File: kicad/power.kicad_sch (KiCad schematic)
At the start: 30 parts, among them J3 Conn_01x02, P1 USB_C_Plug_USB2.0, Q1 BCW66G, Q2 BCW66G, U3 TP4056-42-ESOP8, U4 U8205A, U5 DW01A, U6 USBLC6-2P6, U7 CH340C, U8 AMS1117-3.3

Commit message: init
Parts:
- R10, R11, R12, R3, R4, R5, R6, R7, R8, R9: footprint Resistor_SMD:R_0805_2012Metric -> Resistor_SMD:R_1206_3216Metric
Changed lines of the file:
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@@
 			)
 		)
-		(property "Footprint" "Resistor_SMD:R_0805_2012Metric"
+		(property "Footprint" "Resistor_SMD:R_1206_3216Metric"
 			(at 85.598 163.83 90)
 			(effects
@@
 			)
 		)
-		(property "Footprint" "Resistor_SMD:R_0805_2012Metric"
+		(property "Footprint" "Resistor_SMD:R_1206_3216Metric"
 			(at 105.918 162.56 90)
 			(effects
@@
 			)
 		)
-		(property "Footprint" "Resistor_SMD:R_0805_2012Metric"
+		(property "Footprint" "Resistor_SMD:R_1206_3216Metric"
 			(at 150.368 130.81 90)
 			(effects
@@
 			)
 		)
-		(property "Footprint" "Resistor_SMD:R_0805_2012Metric"
+		(property "Footprint" "Resistor_SMD:R_1206_3216Metric"
 			(at 114.808 154.94 90)
 			(effects
@@
 			)
 		)
-		(property "Footprint" "Resistor_SMD:R_0805_2012Metric"
+		(property "Footprint" "Resistor_SMD:R_1206_3216Metric"
 			(at 105.918 139.7 90)
 			(effects
@@
 			)
 		)
-		(property "Footprint" "Resistor_SMD:R_0805_2012Metric"
+		(property "Footprint" "Resistor_SMD:R_1206_3216Metric"
 			(at 32.258 147.32 90)
 			(effects
@@
 			)
 		)
-		(property "Footprint" "Resistor_SMD:R_0805_2012Metric"
+		(property "Footprint" "Resistor_SMD:R_1206_3216Metric"
 			(at 222.25 79.248 90)
 			(effects
@@
 			)
 		)
-		(property "Footprint" "Resistor_SMD:R_0805_2012Metric"
+		(property "Footprint" "Resistor_SMD:R_1206_3216Metric"
 			(at 221.742 35.56 90)
 			(effects
@@
 			)
 		)
-		(property "Footprint" "Resistor_SMD:R_0805_2012Metric"
+		(property "Footprint" "Resistor_SMD:R_1206_3216Metric"
 			(at 222.25 100.838 90)
 			(effects
@@
 			)
 		)
-		(property "Footprint" "Resistor_SMD:R_0805_2012Metric"
+		(property "Footprint" "Resistor_SMD:R_1206_3216Metric"
 			(at 47.498 147.32 90)
 			(effects

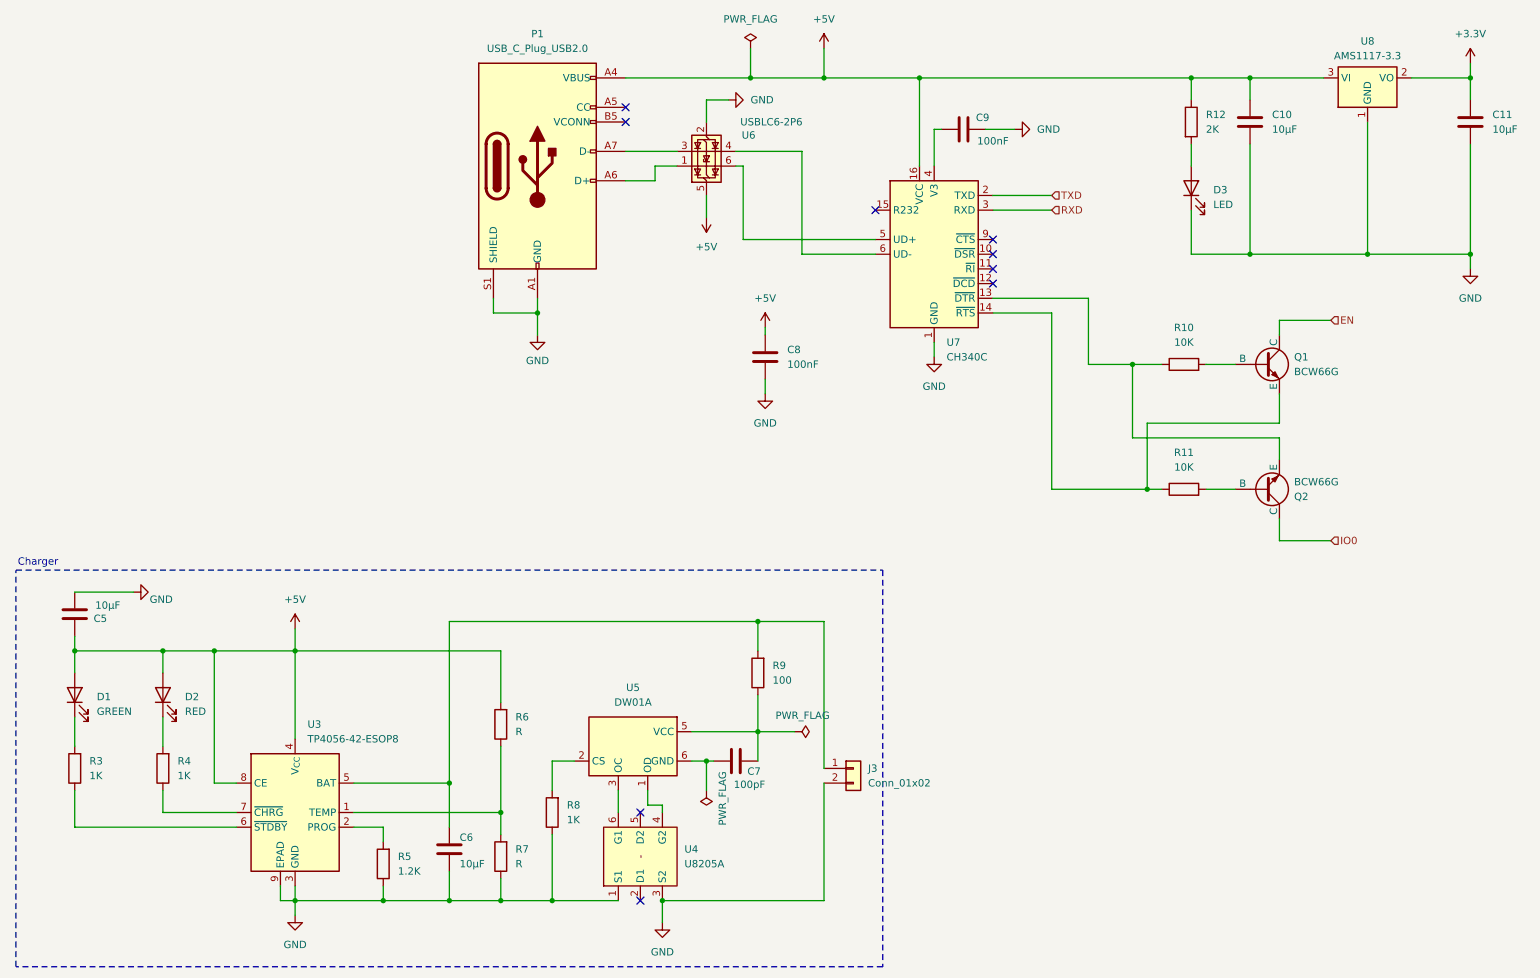
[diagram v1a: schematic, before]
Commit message: init
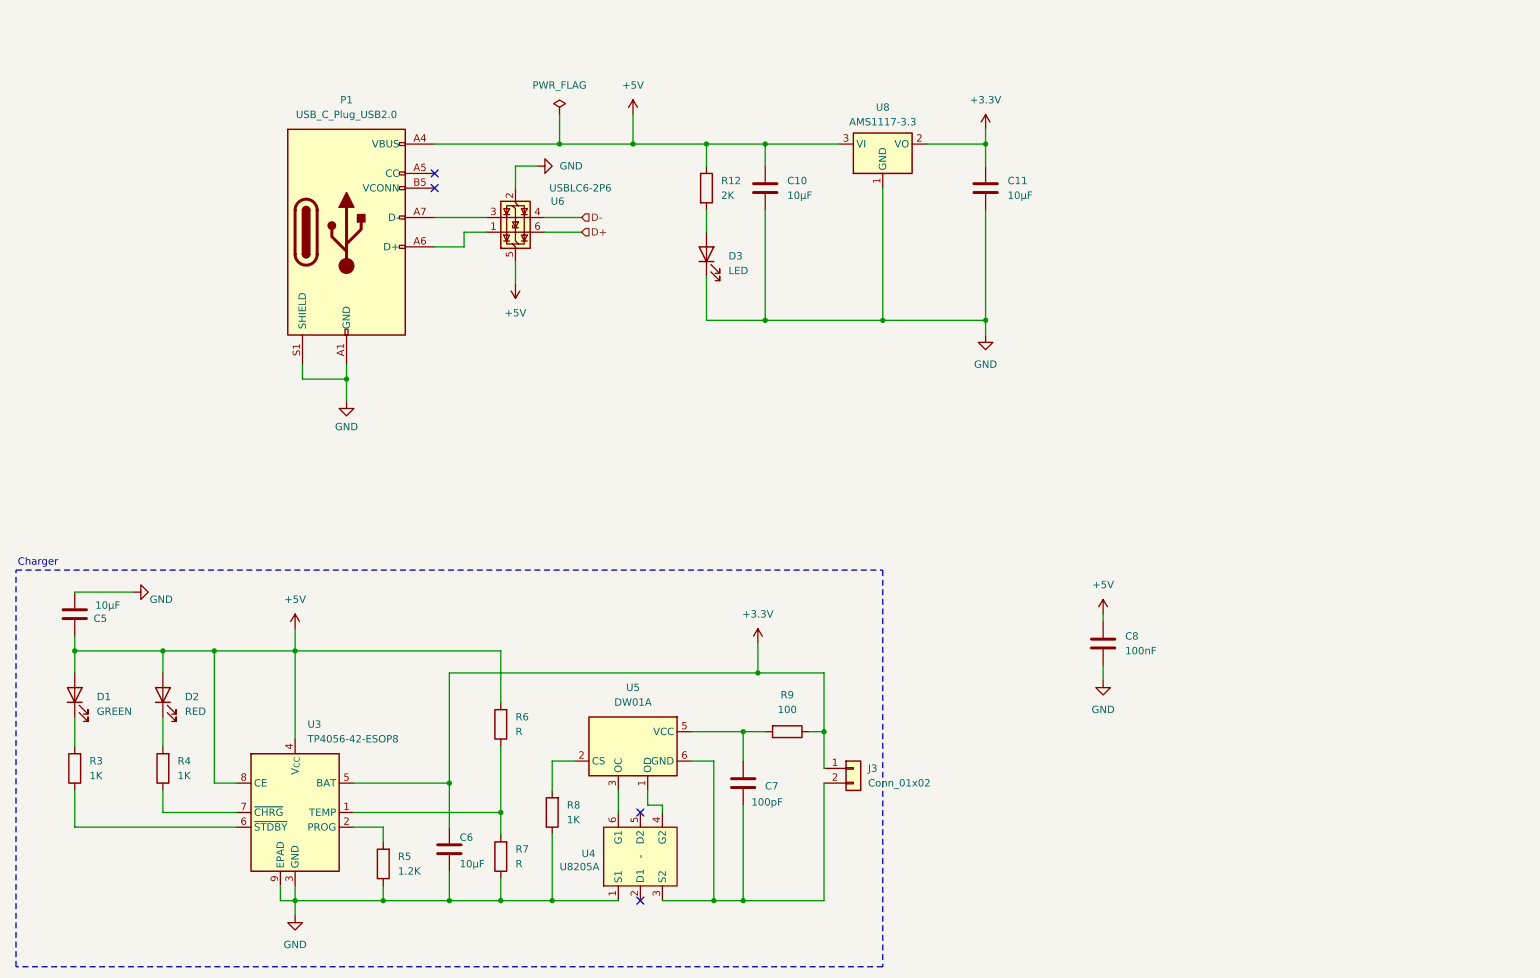
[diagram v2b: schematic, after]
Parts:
- removed C9: 100nF, Capacitor_SMD:C_1206_3216Metric, symbol Device:C
- removed Q1, Q2: BCW66G, Package_TO_SOT_SMD:SOT-23, symbol Simulation_SPICE:NPN
- removed R10, R11: 10K, Resistor_SMD:R_1206_3216Metric, symbol Device:R
- removed U7: CH340C, Package_SO:SOIC-16_3.9x9.9mm_P1.27mm, symbol Interface_USB:CH340C
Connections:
- net +3.3V: now also C6.1, J3.1 (Pin_1), R9.1, U3.5 (BAT)
- net GND: no longer J3.2 (Pin_2), U4.3 (S2)
- net at C7.1, U5.6 (GND): now also J3.2 (Pin_2), U4.3 (S2)
- net at C7.2, U5.5 (VCC): now also R9.2; no longer R9.1
- net D+: now reaches U6.6 (I/O1)
- net D-: now reaches U6.4 (I/O2)
- no-connect marks 9 -> 4
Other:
- moved on the sheet: C10, C11, C7, C8, D3, P1, R12, R9, U6, U8
